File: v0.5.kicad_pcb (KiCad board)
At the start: 2 copper layers, 82 x 38 mm, 65 parts, among them J1 Conn_01x02_Pin, J2 USB_B_Micro, J3 Conn_02x06_Odd_Even, J4 Screw_Terminal_01x08, J5 Screw_Terminal_01x04, J6 Conn_Coaxial_Small, J7 Conn_Coaxial_Small, Q1 MMBT3904, Q2 SiS454DN, Q3 SiS454DN, Q4 SiS454DN, Q5 SiS454DN, U1 MS5611-01BA, U2 L7805, U3 ACS711xLCTR-25AB, U4 ICM-42670-P, U5 SAM-M10Q-0-10, U6 ADXL375BCCZ, U7 Teensy4.1, U8 RFM95W-868S2

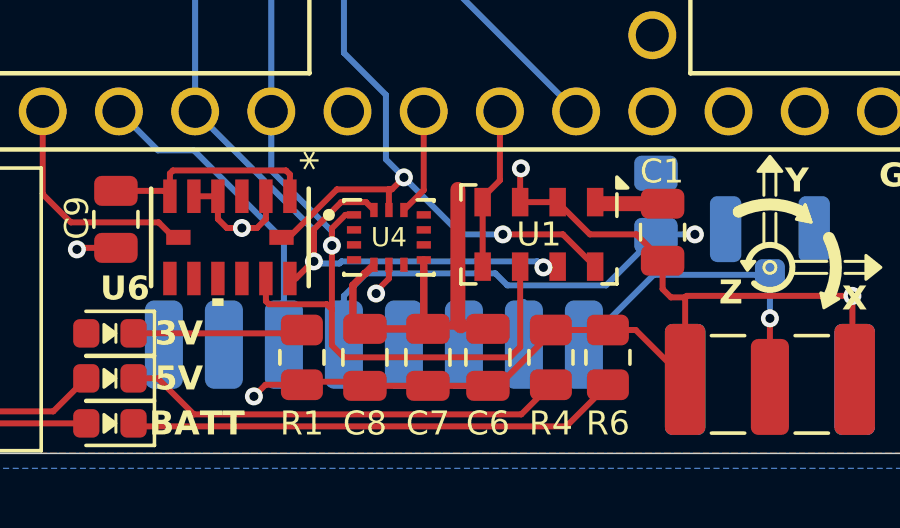
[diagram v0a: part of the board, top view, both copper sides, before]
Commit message: Ready to buy
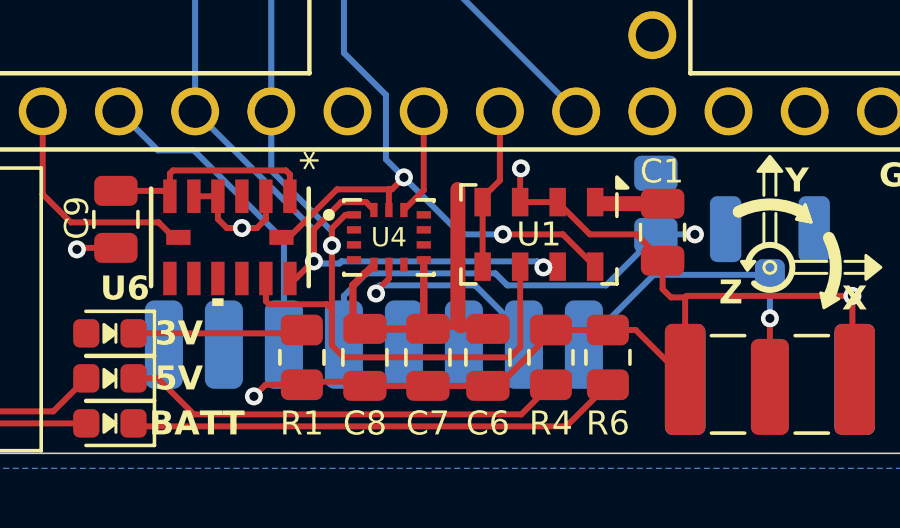
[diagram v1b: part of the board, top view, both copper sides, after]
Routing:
- net GND: track 145.1 -> 149.8 mm
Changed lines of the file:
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@@
 	)
 	(segment
-		(start 146.5 107.35)
-		(end 146.5 108.75)
+		(start 141.7 106.8)
+		(end 144.873278 106.8)
 		(width 0.2)
 		(layer "B.Cu")
+		(net 71)
+	)
+	(segment
+		(start 141.572549 107.07133)
+		(end 141.572549 106.927451)
+		(width 0.2)
+		(layer "B.Cu")
+		(net 71)
+	)
+	(segment
+		(start 146.5 108.426722)
+		(end 146.5 108.775)
+		(width 0.2)
+		(layer "B.Cu")
+		(net 71)
+	)
+	(segment
+		(start 141.572549 106.927451)
+		(end 141.7 106.8)
+		(width 0.2)
+		(layer "B.Cu")
+		(net 71)
+	)
+	(segment
+		(start 144.873278 106.8)
+		(end 146.5 108.426722)
+		(width 0.2)
+		(layer "B.Cu")
